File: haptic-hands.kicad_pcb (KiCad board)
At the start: 2 copper layers, 66.2 x 37.9 mm, 24 parts, among them M1 Motor_DC, SW1 SW_Push, SW2 SW_Push_45deg, SW3 SW_Push_45deg, SW4 SW_Push_45deg, SW5 SW_Push_45deg, SW6 SW_Push_45deg, SW7 SW_Push_45deg, SW8 SW_Push

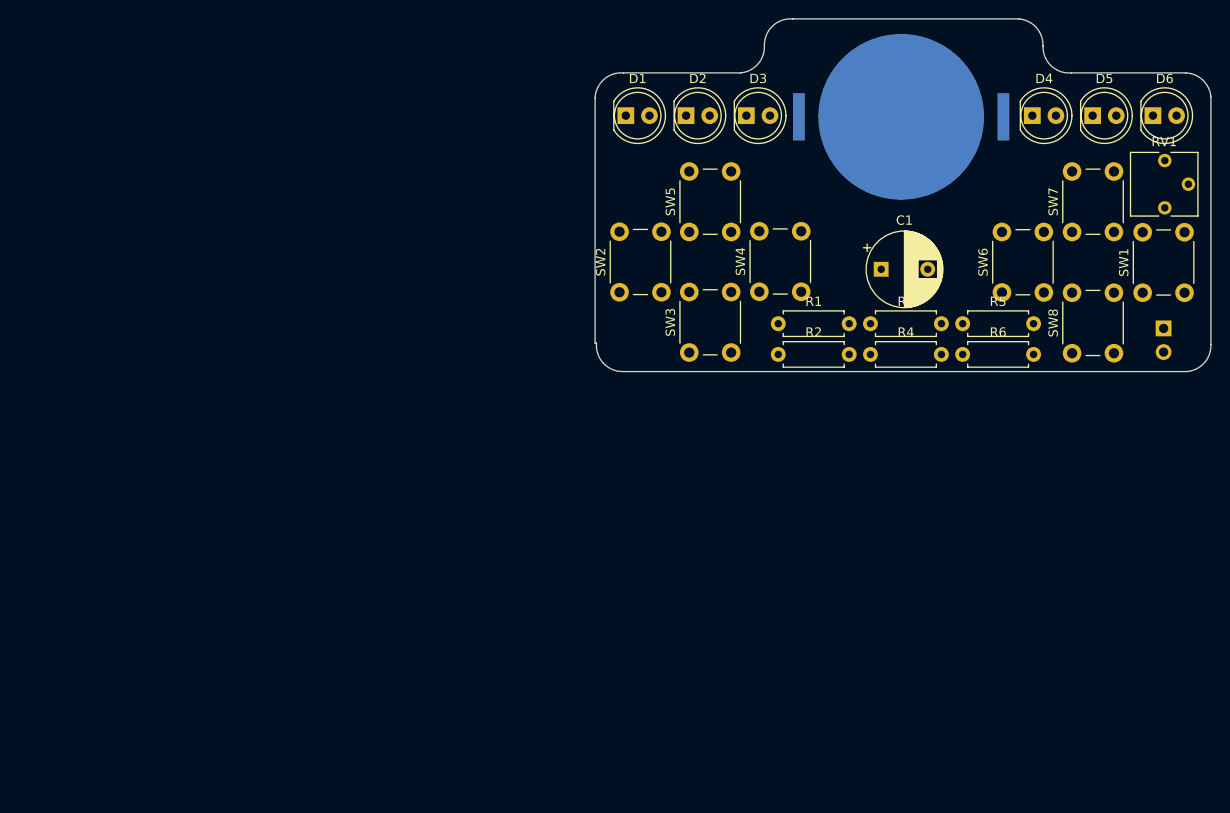
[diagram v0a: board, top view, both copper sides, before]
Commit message: Change layout (again)
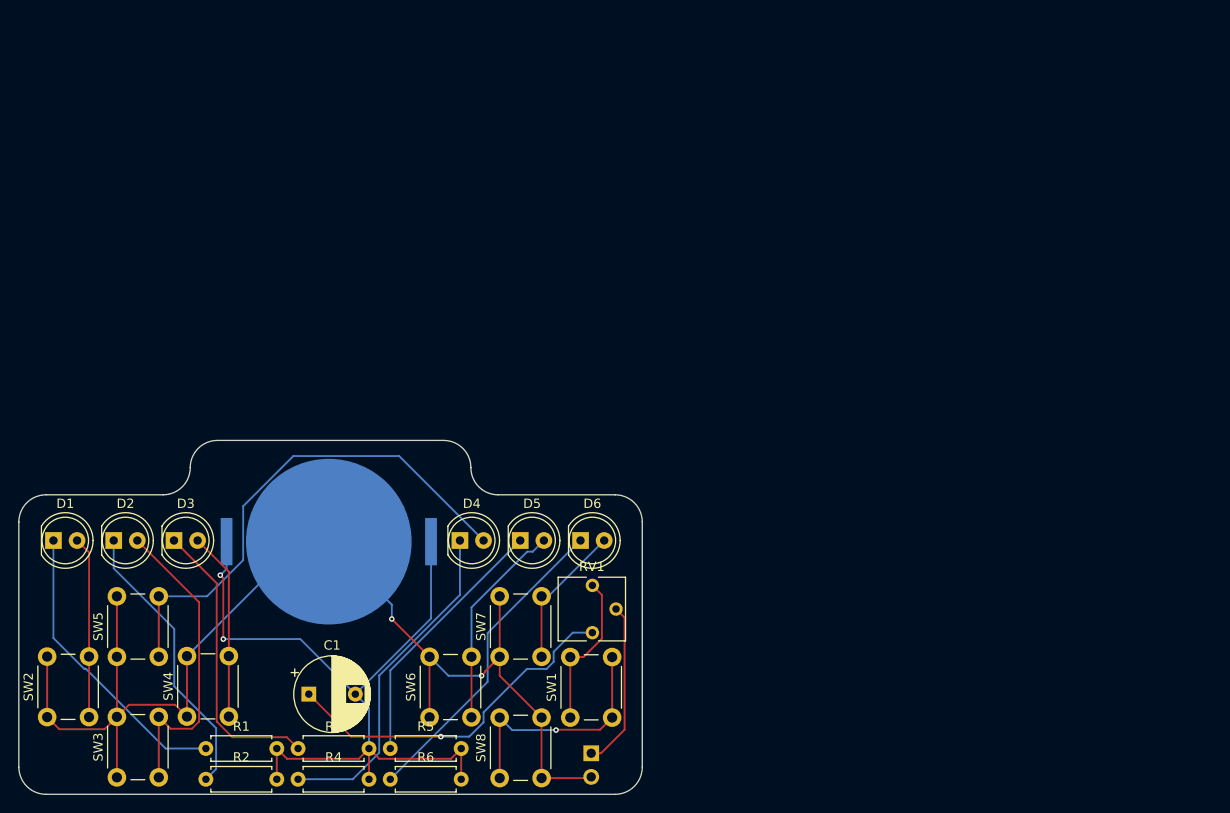
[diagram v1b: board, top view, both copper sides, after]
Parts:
- moved D6 76.6 mm to (103.8, 126.2)
- moved SW6 76.6 mm to (87.6, 145.2)
- moved D1 76.6 mm to (47.2, 126.2)
- moved D2 76.6 mm to (53.7, 126.2)
- moved D3 76.6 mm to (60.1, 126.2)
- moved D4 76.6 mm to (90.9, 126.2)
- moved D5 76.6 mm to (97.3, 126.2)
- moved M1 76.6 mm to (105.0, 149.1)
- moved R1 76.6 mm to (63.6, 148.6)
- moved R2 76.6 mm to (63.6, 151.9)
- moved R3 76.6 mm to (73.5, 148.6)
- moved R4 76.6 mm to (73.5, 151.9)
- moved R5 76.6 mm to (83.4, 148.6)
- moved R6 76.6 mm to (83.4, 151.9)
- moved RV1 76.6 mm to (105.1, 136.1)
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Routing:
- net Net-(BT1--): track 0.00 -> 129.4 mm, vias 0 -> 2
- net Net-(BT1-+): track 0.00 -> 85.3 mm, vias 0 -> 2
- net Net-(D4-A): track 0.00 -> 54.8 mm
- net Net-(C1-Pad1): track 0.00 -> 38.2 mm, vias 0 -> 1
- net Net-(D4-K): track 0.00 -> 36.3 mm
- net Net-(D6-K): track 0.00 -> 34.1 mm
- net Net-(D2-A): track 0.00 -> 33.9 mm
- net Net-(D1-K): track 0.00 -> 31.8 mm
- net Net-(D3-K): track 0.00 -> 31.3 mm
- net Net-(D2-K): track 0.00 -> 30.7 mm
- net Net-(D5-K): track 0.00 -> 28.1 mm
- net Net-(SW1-Pad2): track 0.00 -> 26.2 mm, vias 0 -> 1
- net Net-(D5-A): track 0.00 -> 22.6 mm
- net Net-(D3-A): track 0.00 -> 20.3 mm
- net Net-(D1-A): track 0.00 -> 19.5 mm
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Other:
- board size 66.2 x 37.9 mm -> 67 x 38 mm
